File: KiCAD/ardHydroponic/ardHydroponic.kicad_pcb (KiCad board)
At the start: 2 copper layers, 102.9 x 54.6 mm, 4 parts, among them U10 ESP-01

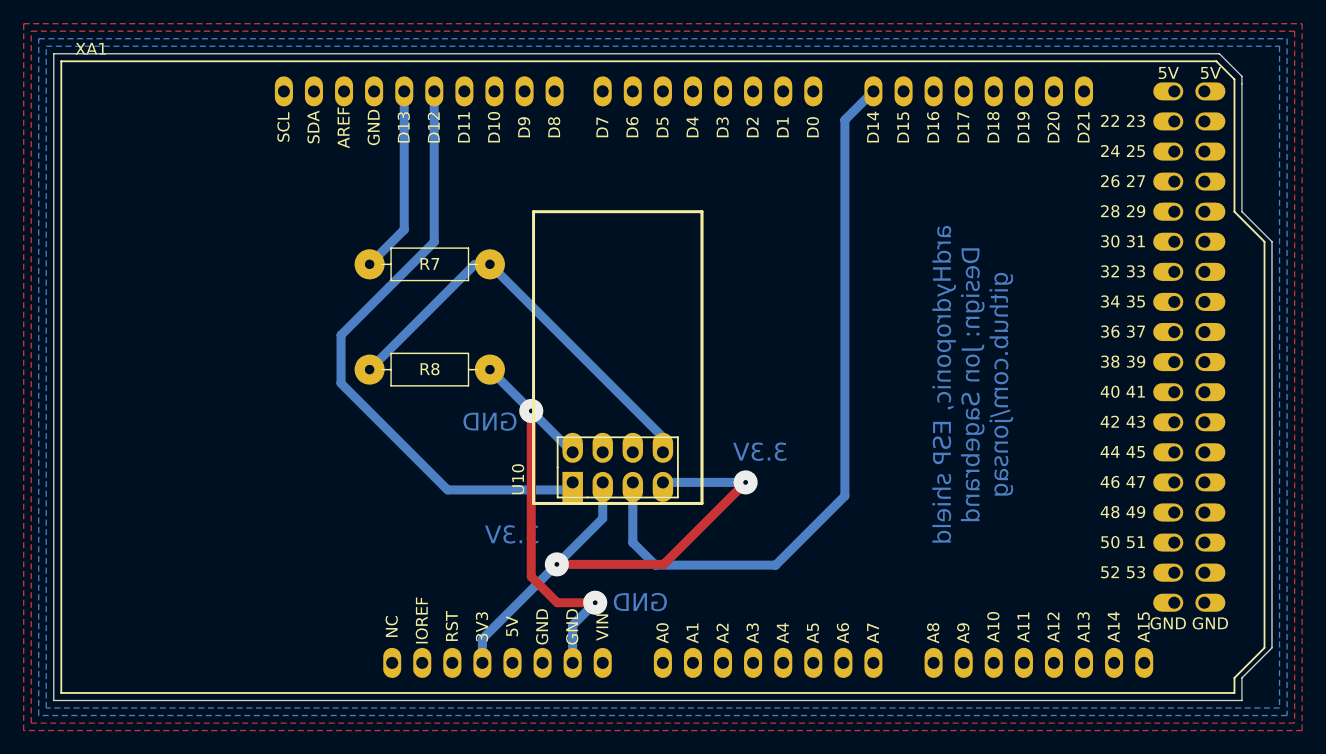
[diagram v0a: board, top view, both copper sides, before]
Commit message: pcb layout
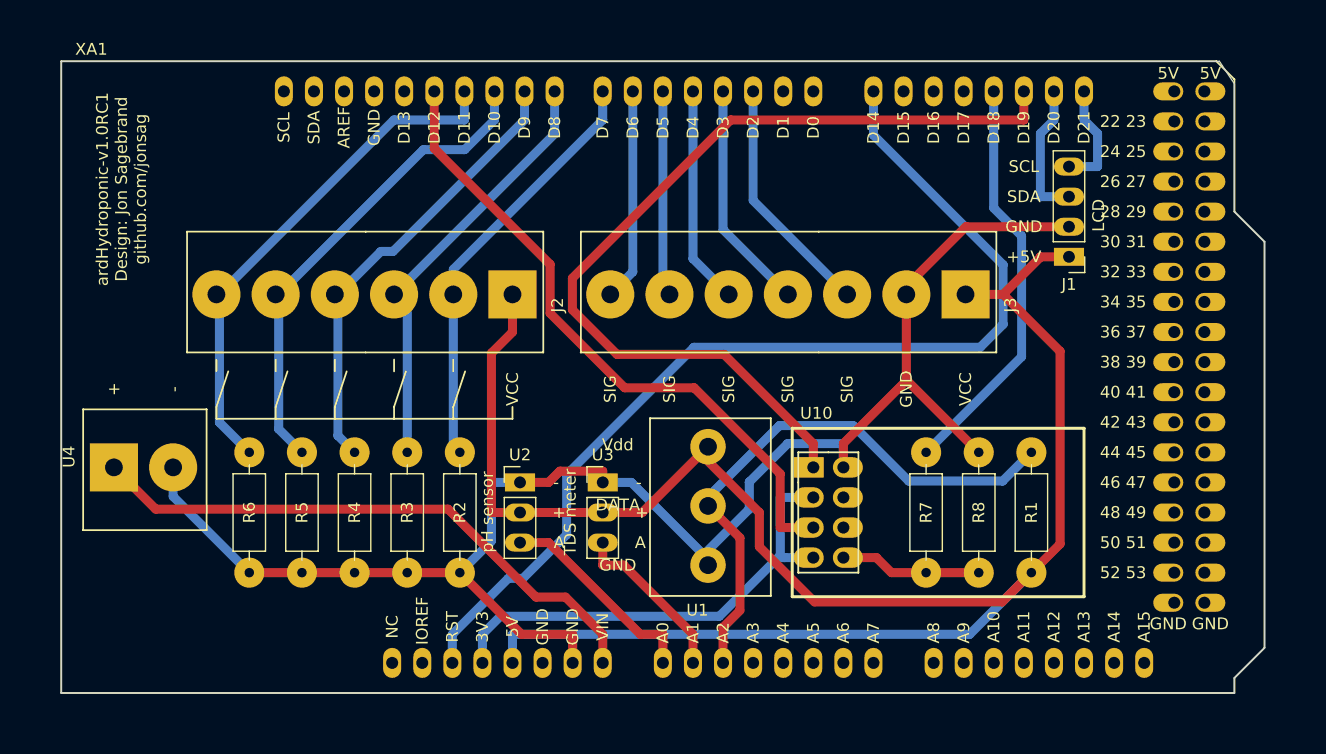
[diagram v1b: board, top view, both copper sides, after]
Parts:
- added J1: LCD display, My_Headers:4-pin_I2C_LCD_header_larger, F.Cu at (185.4, 87.6)
- added J2: Buttons, My_Parts:6-pole_5-NO_switch_screw_terminal, F.Cu at (138.4, 90.8)
- added J3: MOSFETs, My_Parts:7-pole_6-MOSFET_screw_terminal, F.Cu at (176.7, 90.8)
- added R1: 4.7k, My_Misc:R_Axial_DIN0207_L6.3mm_D2.5mm_P10.16mm_Horizontal_larger_pads, F.Cu at (182.2, 104.1)
- added R2: 10k, My_Misc:R_Axial_DIN0207_L6.3mm_D2.5mm_P10.16mm_Horizontal_larger_pads, F.Cu at (134.0, 114.3)
- added R3: 10k, My_Misc:R_Axial_DIN0207_L6.3mm_D2.5mm_P10.16mm_Horizontal_larger_pads, F.Cu at (129.5, 114.3)
- added R4: 10k, My_Misc:R_Axial_DIN0207_L6.3mm_D2.5mm_P10.16mm_Horizontal_larger_pads, F.Cu at (125.1, 114.3)
- added R5: 10k, My_Misc:R_Axial_DIN0207_L6.3mm_D2.5mm_P10.16mm_Horizontal_larger_pads, F.Cu at (120.7, 114.3)
- added R6: 10k, My_Misc:R_Axial_DIN0207_L6.3mm_D2.5mm_P10.16mm_Horizontal_larger_pads, F.Cu at (116.2, 114.3)
- added U1: DS18B20, My_Parts:3-pole_DS18B20_screw_terminal, F.Cu at (154.9, 113.7)
- added U2: pH sensor, My_Headers:3-pin_DFRobot_Gravity_pH-sensor_header_large, F.Cu at (139.1, 106.7)
- added U3: TDS meter, My_Headers:3-pin_DFRobot_Gravity_TDS-meter_header_large, F.Cu at (146.1, 106.7)
- added U4: Power in, My_Parts:2-pole_power_in_screw_terminal, F.Cu at (104.8, 105.4)
- moved R8 54.2 mm to (177.8, 114.3), turned to 90 degrees
- moved R7 49.6 mm to (173.4, 104.1), turned to 270 degrees
- moved U10 20.4 mm to (163.8, 105.4), turned to 0 degrees
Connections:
- R7 pad 1: softTx -> Tx
- U10 pad 1: softRx -> Rx
- XA1 pad 100: +6V -> Net-(U4-Pad1)
- XA1 pad 25: softRx -> espReset
- XA1 pad 26: softTx -> Net-(XA1-Pad26)
- XA1 pad 45: Net-(XA1-Pad45) -> Rx
- XA1 pad 46: Net-(XA1-Pad46) -> Tx
- XA1 pad 64: espReset -> Net-(XA1-Pad30)
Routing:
- net +5V: track 0.00 -> 160.5 mm
- net GND: track 36.0 -> 136.0 mm, vias 2 -> 0
- net Net-(XA1-Pad30): track 0.00 -> 86.9 mm
- net Rx: track 0.00 -> 75.8 mm
- net softRx: track 51.2 -> 0.00 mm
- net Net-(U4-Pad1): track 0.00 -> 49.5 mm
- net Net-(R1-Pad1): track 0.00 -> 48.5 mm
- net button5: track 0.00 -> 43.8 mm
- net button4: track 0.00 -> 41.1 mm
- net button3: track 0.00 -> 38.5 mm
- net button2: track 0.00 -> 36.6 mm
- net button1: track 0.00 -> 35.9 mm
- net Tx: track 0.00 -> 34.8 mm
- net Net-(R7-Pad2): track 35.1 -> 12.0 mm
- net pH+: track 0.00 -> 20.4 mm
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- removed copper zone on B.Cu, net (none)
- removed copper zone on F.Cu, net (none)
- removed copper zone on B.Cu, net GND
- removed copper zone on F.Cu, net GND
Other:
- board size 102.9 x 54.6 mm -> 101.6 x 53.3 mm
- board text added: "ardHydroponic-v1.0RC1 Design: Jon Sagebrand github.com/jonsag"
- board text removed: "3.3V"
- board text removed: "GND"
- board text removed: "ardHydroponic, ESP shield Design: Jon Sagebrand github.com/jonsag"
